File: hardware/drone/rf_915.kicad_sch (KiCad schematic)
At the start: 1 part, among them U2 SX1262IMLTRT

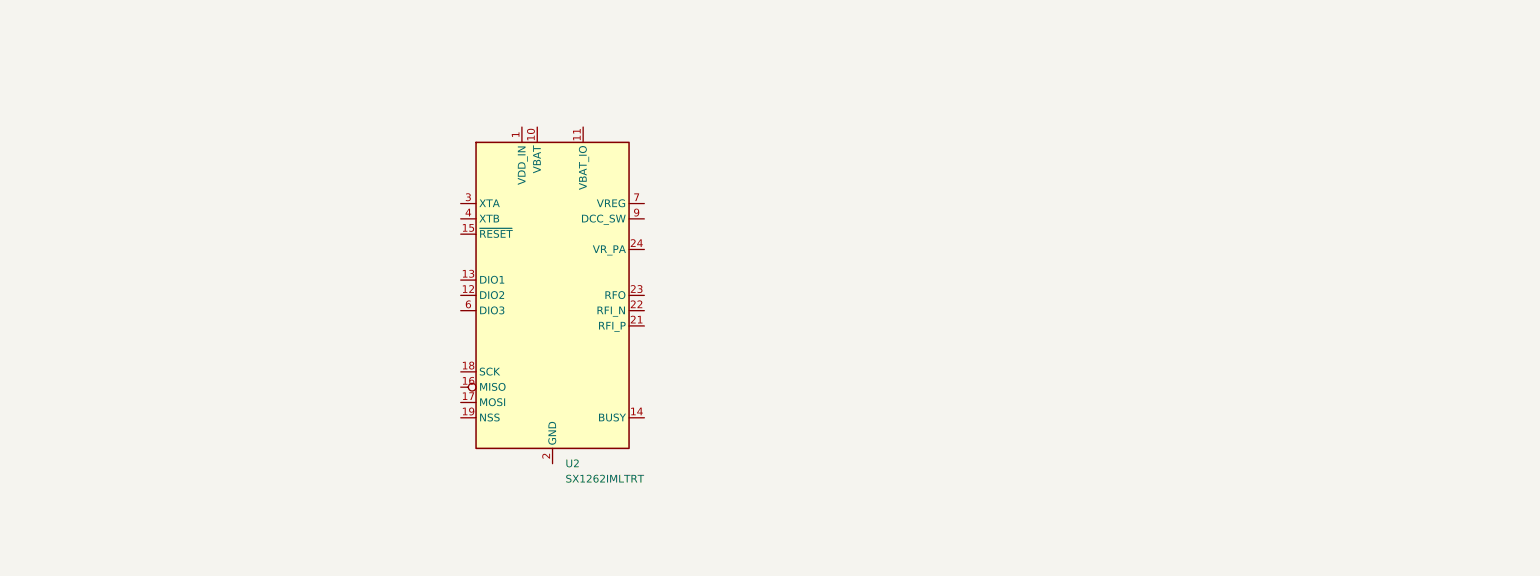
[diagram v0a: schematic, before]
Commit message: more radio work
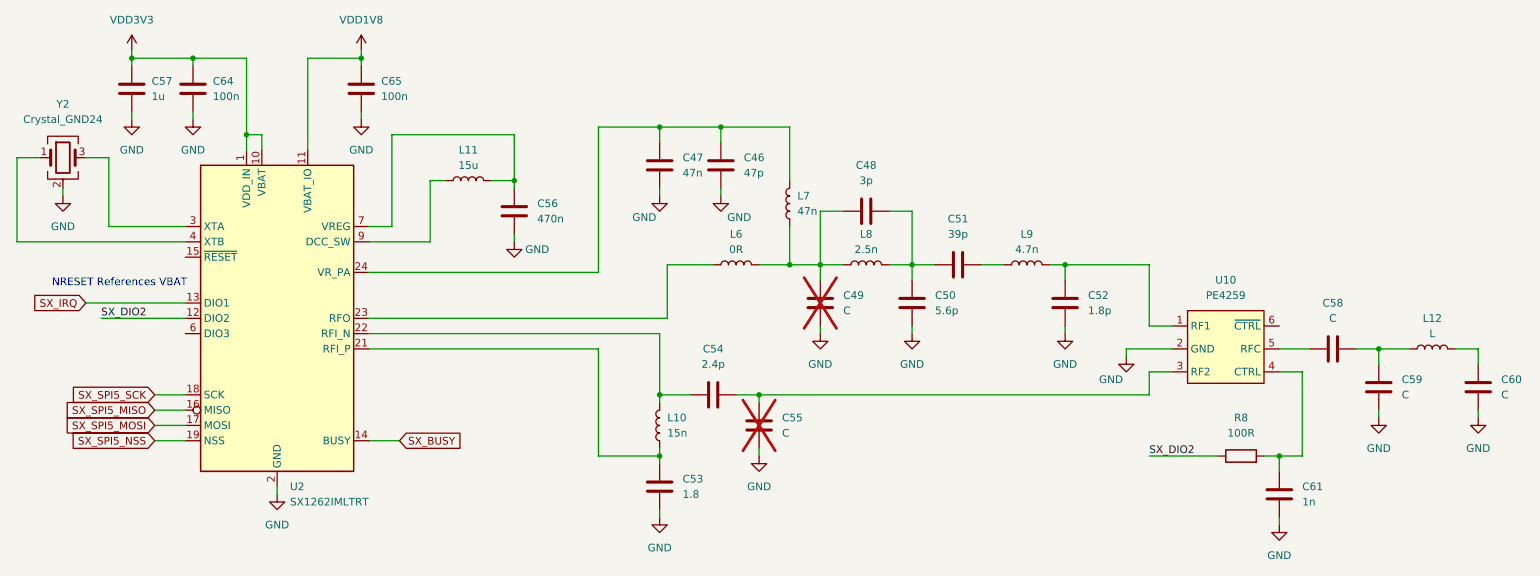
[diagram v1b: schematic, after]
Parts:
- added C46: 47p, symbol Device:C
- added C47: 47n, symbol Device:C
- added C48: 3p, symbol Device:C
- added C49, C55, C58, C59, C60: C, symbol Device:C
- added C50: 5.6p, symbol Device:C
- added C51: 39p, symbol Device:C
- added C52: 1.8p, symbol Device:C
- added C53: 1.8, symbol Device:C
- added C54: 2.4p, symbol Device:C
- added C56: 470n, symbol Device:C
- added C57: 1u, symbol Device:C
- added C61: 1n, symbol Device:C
- added C64, C65: 100n, symbol Device:C
- added L10: 15n, symbol Device:L
- added L11: 15u, symbol Device:L
- added L12: L, symbol Device:L
- added L6: 0R, symbol Device:L
- added L7: 47n, symbol Device:L
- added L8: 2.5n, symbol Device:L
- added L9: 4.7n, symbol Device:L
- added R8: 100R, symbol Device:R
- added U10: PE4259, symbol SoftDrone:PE4259
- added Y2: Crystal_GND24, symbol Device:Crystal_GND24
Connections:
- net VDD3V3: now reaches U2.1 (VDD_IN)
- net VDD3V3: now also U2.10 (VBAT), C57.1, C64.1
- net VDD1V8: now reaches U2.11 (VBAT_IO)
- net VDD1V8: now also C65.1
- net SX_DIO2: now reaches U2.12 (DIO2)
- net SX_DIO2: now also R8.1
- net SX_IRQ: now reaches U2.13 (DIO1)
- net SX_BUSY: now reaches U2.14 (BUSY)
- net SX_SPI5_MISO: now reaches U2.16 (MISO)
- net SX_SPI5_MOSI: now reaches U2.17 (MOSI)
- net SX_SPI5_SCK: now reaches U2.18 (SCK)
- net SX_SPI5_NSS: now reaches U2.19 (NSS)
- net GND: now reaches U2.2 (GND), U2.20 (GND), U2.25 (GND), U2.5 (GND), U2.8 (GND)
- net GND: now also C46.2, C47.2, C49.2, C50.2, C52.1, C53.1, C55.2, C56.2, C57.2, C59.1, C60.1, C61.1, C64.2, C65.2, U10.2 (GND), Y2.2 (G), Y2.4 (G)
- net at U2.21 (RFI_P): now also C53.2, L10.1
- net at U2.22 (RFI_N): now also C54.2, L10.2
- net at U2.23 (RFO): now also L6.1
- net at U2.24 (VR_PA): now also C46.1, C47.1, L7.2
- net at U2.3 (XTA): now also Y2.3
- net at U2.4 (XTB): now also Y2.1
- net at U2.7 (VREG): now also C56.1, L11.2
- net at U2.9 (DCC_SW): now also L11.1
- new net: C61.2, R8.2, U10.4 (CTRL)
- new net: C54.1, C55.1, U10.3 (RF2)
- new net: C48.1, C49.1, L6.2, L7.1, L8.1
- new net: C58.2, C59.2, L12.1
- new net: C60.2, L12.2
- new net: C48.2, C50.1, C51.1, L8.2
- new net: C51.2, L9.1
- new net: C52.2, L9.2, U10.1 (RF1)
- new net: C58.1, U10.5 (RFC)
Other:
- note added: "NRESET References VBAT"
- moved on the sheet: U2
